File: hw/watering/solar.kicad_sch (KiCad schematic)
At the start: 24 parts, among them U2 DRV8220DSG, U5 STI3508

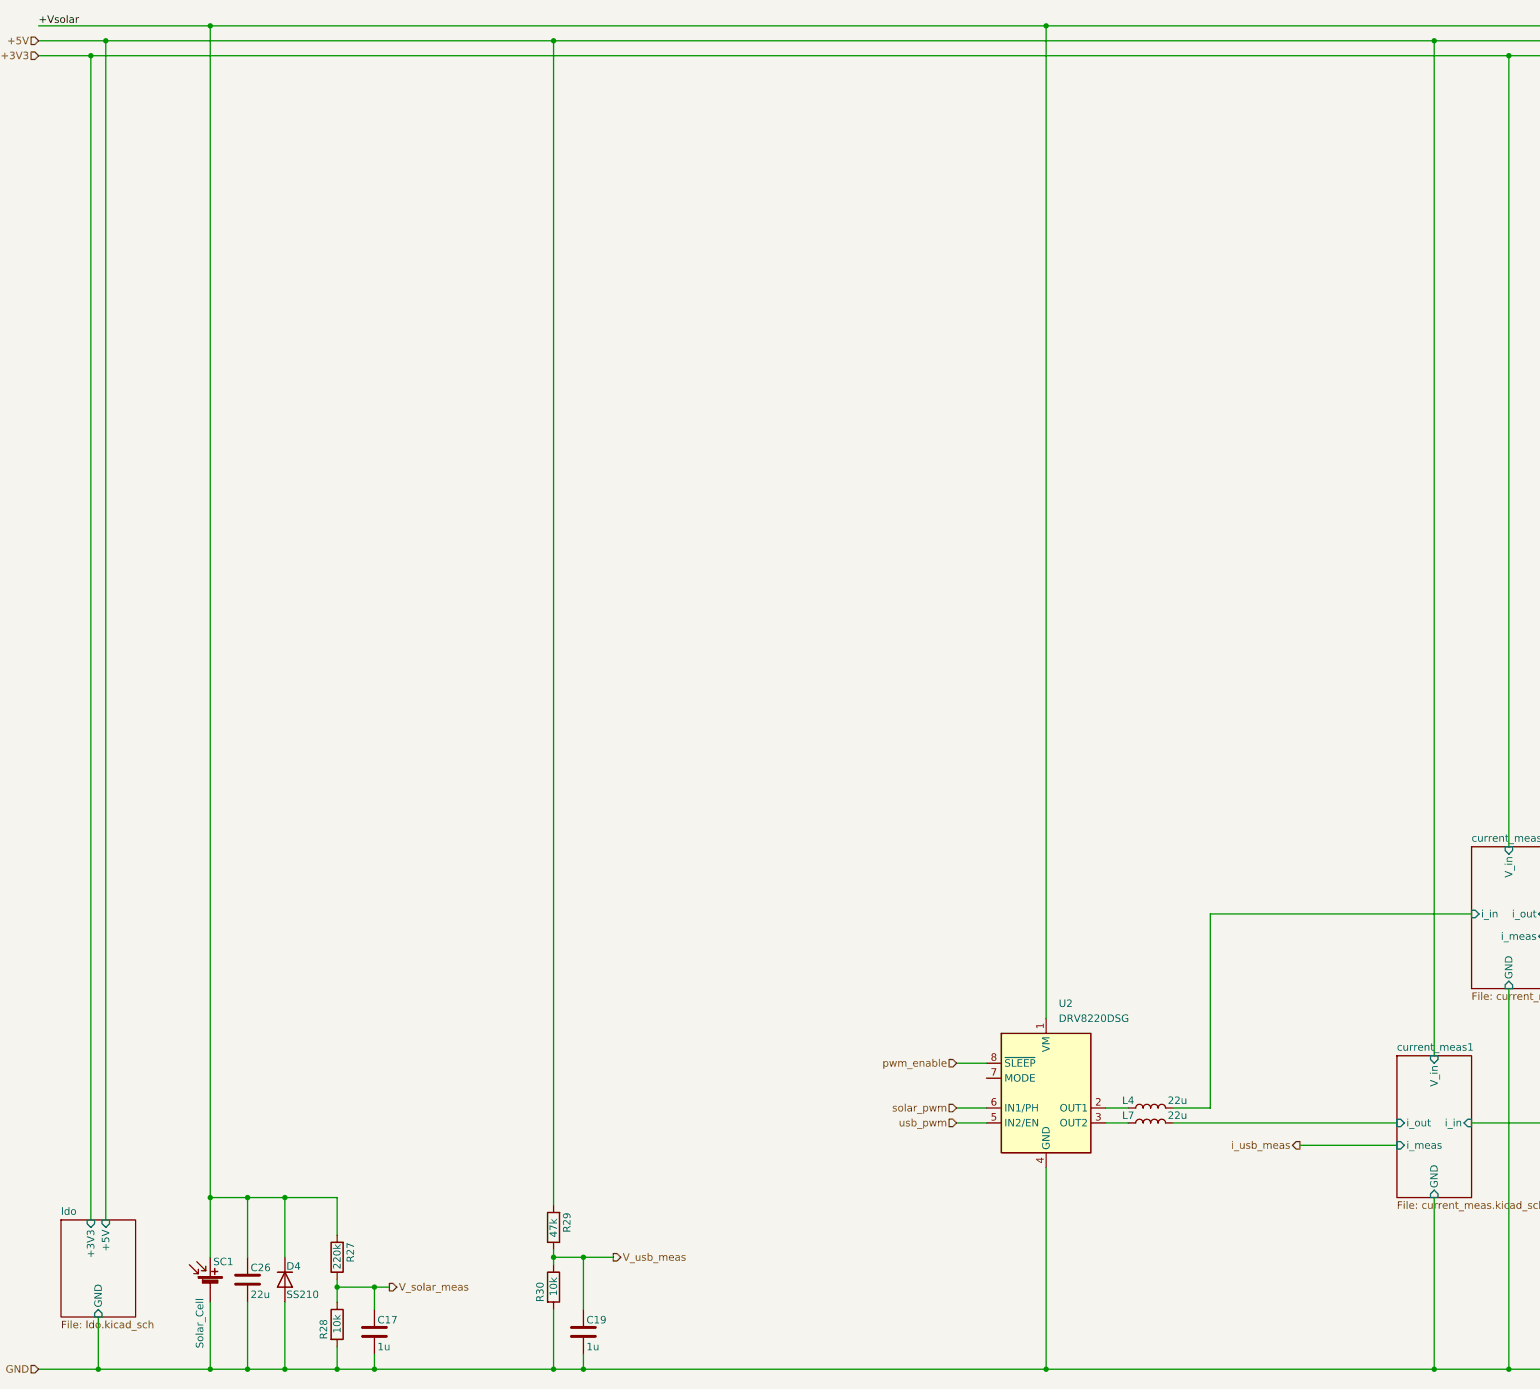
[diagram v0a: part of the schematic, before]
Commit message: routing done
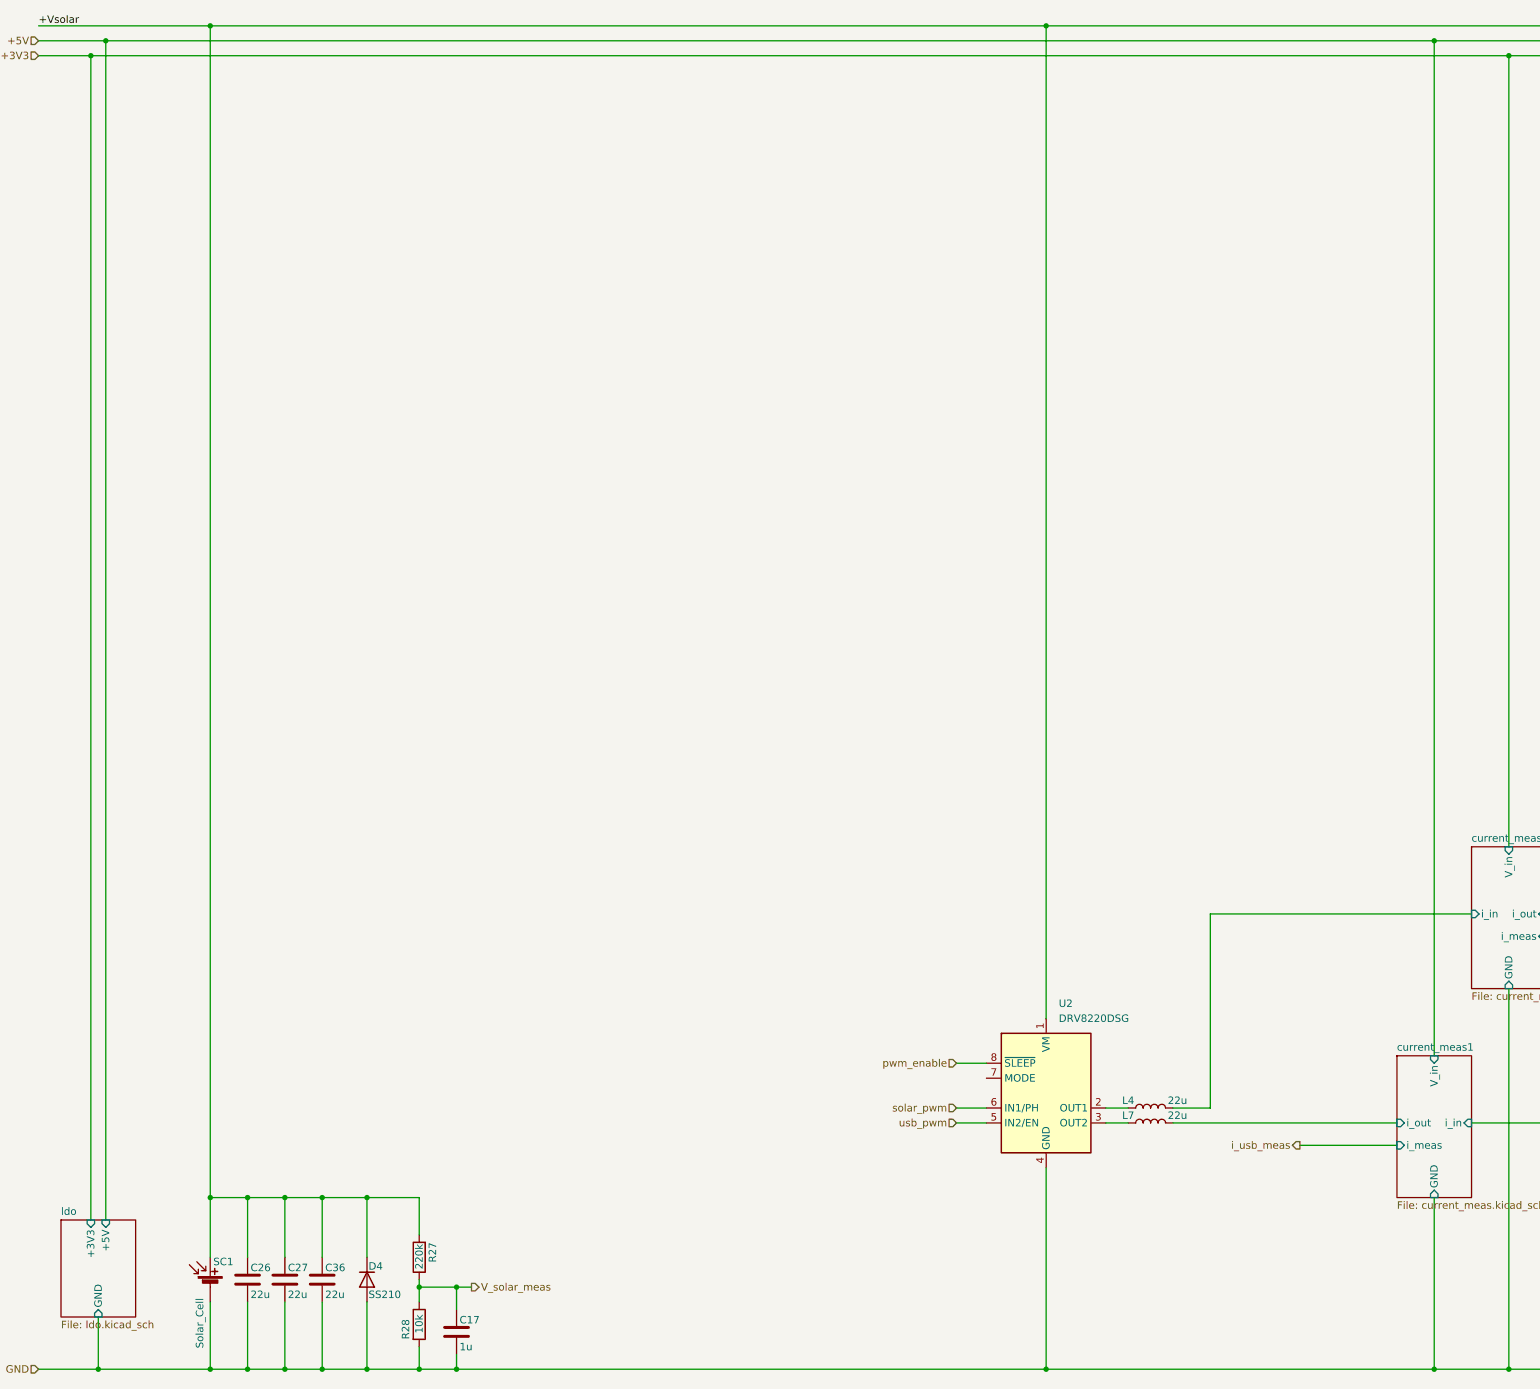
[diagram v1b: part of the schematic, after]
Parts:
- removed C19: 1u, Capacitor_SMD:C_0603_1608Metric, symbol Device:C
- removed R29: 47k, Resistor_SMD:R_0603_1608Metric, symbol Device:R
- removed R30: 10k, Resistor_SMD:R_0603_1608Metric, symbol Device:R
- added C27, C36: 22u, Capacitor_SMD:C_1206_3216Metric, symbol Device:C
- SC1: footprint Capacitor_THT:CP_Axial_L20.0mm_D10.0mm_P26.00mm_Horizontal -> DORABO:DB142R-5.08-2P-GN
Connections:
- net +Vsolar: now also C27.1, C36.1
- net GND: now also C27.2, C36.2
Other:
- moved on the sheet: C17, D4, R27, R28
